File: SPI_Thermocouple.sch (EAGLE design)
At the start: 7 parts, among them U1 MAX31855

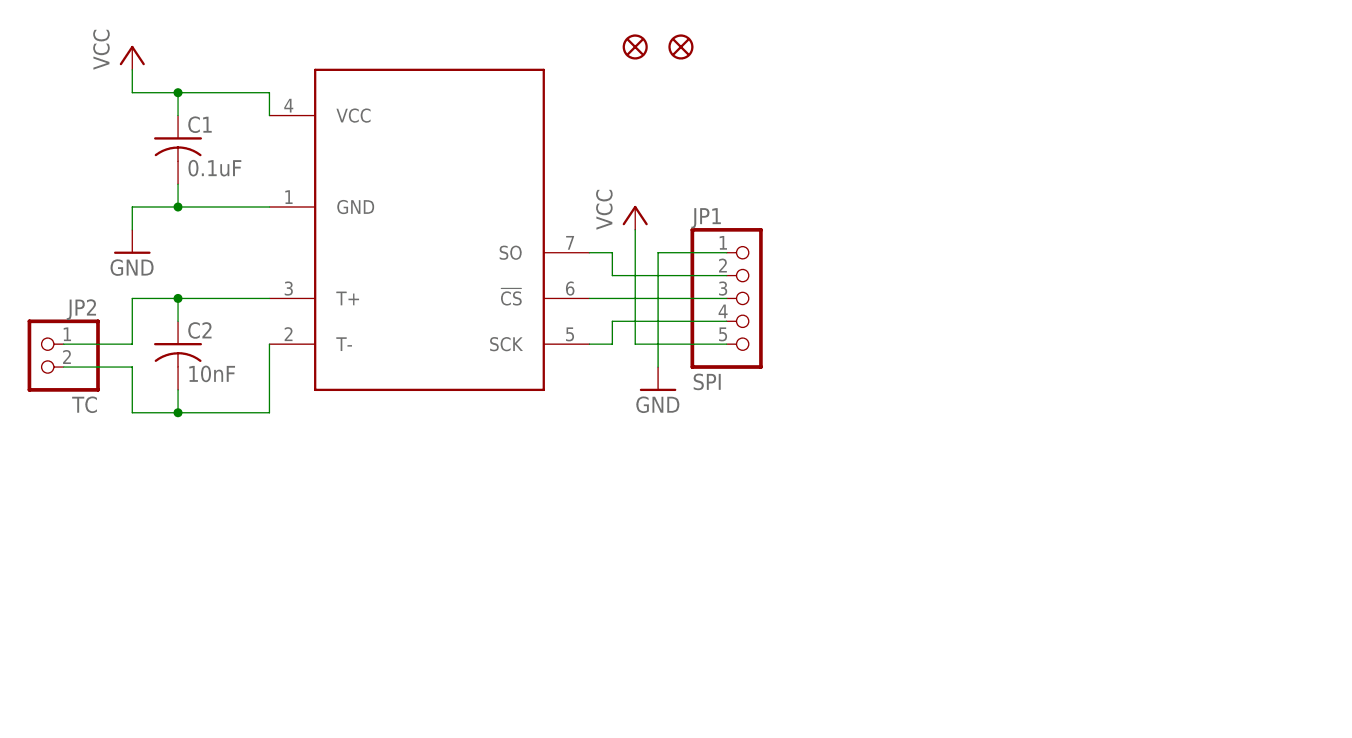
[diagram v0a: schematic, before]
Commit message: upgrade design to a wing
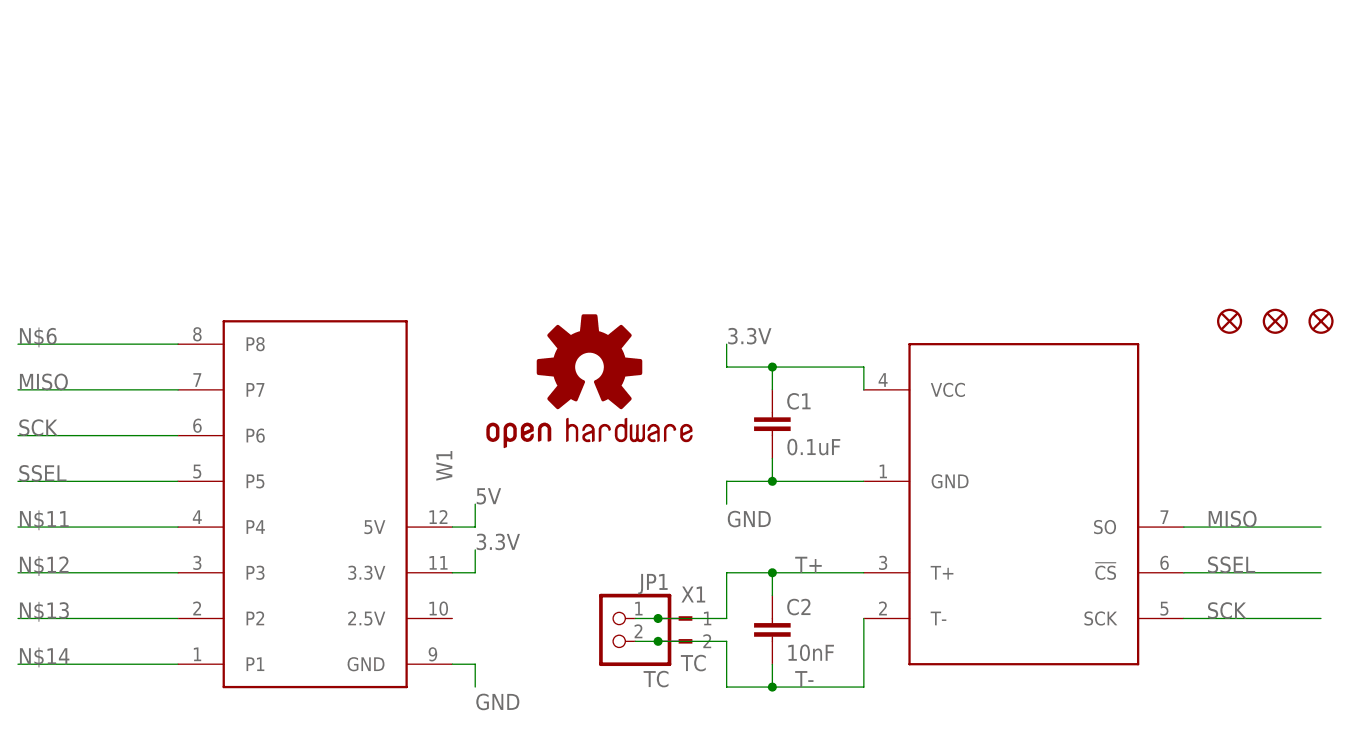
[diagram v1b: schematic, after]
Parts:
- removed JP2: TC, pinhead:PINHD-1X2
- removed JP3, JP4: FIDUCIAL1X2, SparkFun:FIDUCIAL1X2
- added FID1, FID2, FID3: FIDUCIAL1X2, SparkFun:FIDUCIAL1X2
- added U$1: OSHW-LOGOS, logxen:OSHW-LOGOS
- added W1: PAPILIO-WING-8BITS, logxen:PAPILIO-WING-8BITS
- added X1: TC, con-weidmueller-sl35:180-2
- C1: device resistor:C-USC1206 -> SparkFun-Passives:CAP1206
- C2: device resistor:C-USC1206 -> SparkFun-Passives:CAP0603-CAP
- JP1: value SPI -> TC; device pinhead:PINHD-1X5 -> pinhead:PINHD-1X2
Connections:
- removed net N$1: C2.1, JP2.1, U1.T+
- removed net N$2: C2.2, JP2.2, U1.T-
- removed net N$3: JP1.3, U1.!CS
- removed net N$4: JP1.2, U1.SO
- removed net N$5: JP1.4, U1.SCK
- removed net VCC: C1.1, JP1.5, U1.VCC
- new net 3.3V: C1.1, U1.VCC, W1.3.3V
- new net 5V: W1.5V
- new net MISO: U1.SO, W1.P7
- new net N$11: W1.P4
- new net N$12: W1.P3
- new net N$13: W1.P2
- new net N$14: W1.P1
- new net N$6: W1.P8
- new net SCK: U1.SCK, W1.P6
- new net SSEL: U1.!CS, W1.P5
- new net T+: C2.1, JP1.1, U1.T+, X1.1
- new net T-: C2.2, JP1.2, U1.T-, X1.2
- net GND: now also W1.GND; no longer JP1.1
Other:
- moved on the sheet: C1, C2
